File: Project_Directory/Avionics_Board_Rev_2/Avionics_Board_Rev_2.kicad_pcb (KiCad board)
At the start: 2 copper layers, 60.1 x 130 mm, 87 parts, among them J1 Battery, J10 PWM_1, J11 PWM_2, J12 PWM_3, J13 I2C, J14 UART, J15 Conn_Coaxial, J16 ON, J2 ARM, J3 PYRO_1, J4 PYRO_3, J5 PYRO_2, J6 PYRO_4, J7 PWM_4, J8 PWM_5, J9 PWM_6, Q1 Drive_MOS, Q2 Drive_MOS, Q3 Drive_MOS, Q4 Drive_MOS, Q5 Drive_MOS, SW1 SW_DPDT_x2, U1 Teensy4.1, U10 GSM, U11 AP2127K-3.3, U2 LoRa - RFM95-W/PW, U3 ADXL, U4 ADS1115IDGS, U5 AMS1117-3.3, U6 GPS, U7 GY-91, U8 AMS1117-5.0

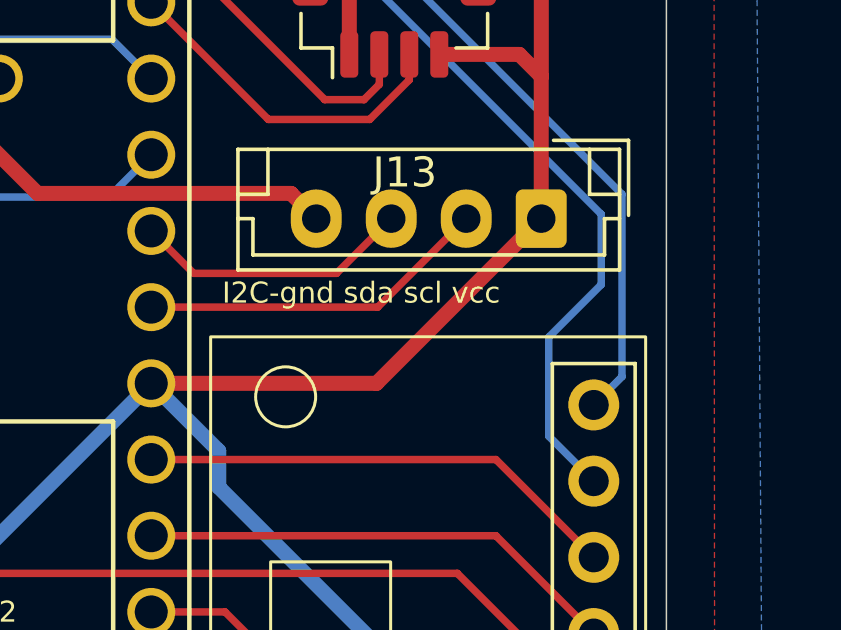
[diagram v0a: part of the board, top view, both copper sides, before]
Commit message: Modification 3 7th march
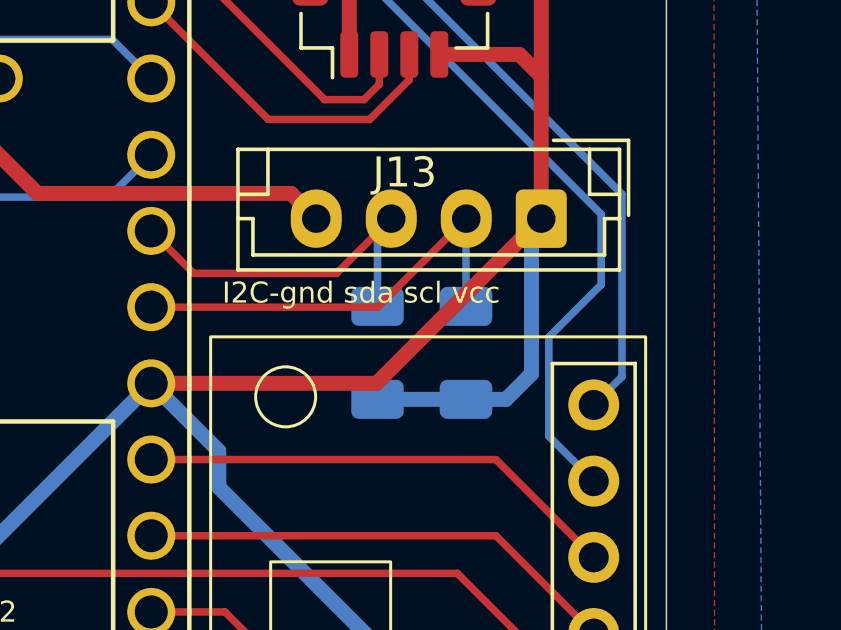
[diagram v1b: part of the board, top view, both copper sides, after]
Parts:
- added R27: 2.2k, Resistor_SMD:R_1206_3216Metric_Pad1.30x1.75mm_HandSolder, B.Cu at (173.2, 59.5)
- added R28: 2.2k, Resistor_SMD:R_1206_3216Metric_Pad1.30x1.75mm_HandSolder, B.Cu at (176.2, 59.5)
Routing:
- net +3.3V: track 211.8 -> 222.6 mm
- net /Spare_I2C_SDA: track 9.34 -> 12.5 mm
- net /Spare_I2C_SCL: track 11.7 -> 14.6 mm
